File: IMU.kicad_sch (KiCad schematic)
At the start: 0 parts

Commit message: new update
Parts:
- added C29, C30: 100nF, C0402C104K4RAC:CAPC1005X55N, symbol C0402C104K4RAC:C0402C104K4RAC
- added U1: BMI088, Module:PQFN50P450X300X100-16N, symbol BMI088:BMI088
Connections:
- new net +3V3_BMI: C29.2, C30.2, U1.11 (VDDIO), U1.3 (VDD)
- new net CSB_ACCEL: U1.14 (CSB1)
- new net CSB_GYRO: U1.5 (CSB2)
- new net GND: C29.1, C30.1, U1.2 (NC), U1.4 (GNDA), U1.6 (GNDIO), U1.7 (PS)
- new net INT1_ACCEL: U1.16 (INT1)
- new net INT1_GYRO: U1.12 (INT3)
- new net INT2_ACCEL: U1.1 (INT2)
- new net INT2_GYRO: U1.13 (INT4)
- new net MISO: U1.10 (SDO2), U1.15 (SDO1)
- new net MOSI: U1.9 (SDA/SDI)
- new net SCK: U1.8 (SCL/SCK)

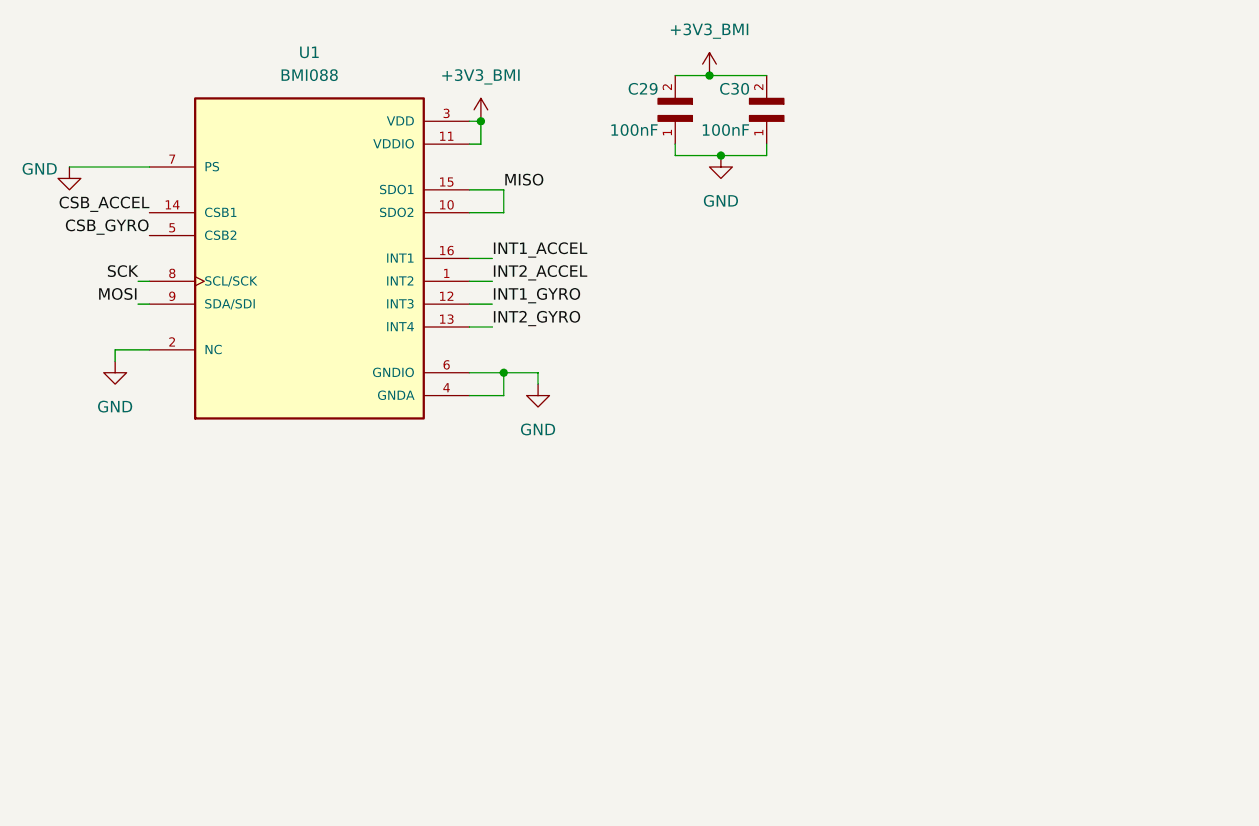
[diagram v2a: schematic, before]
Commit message: new
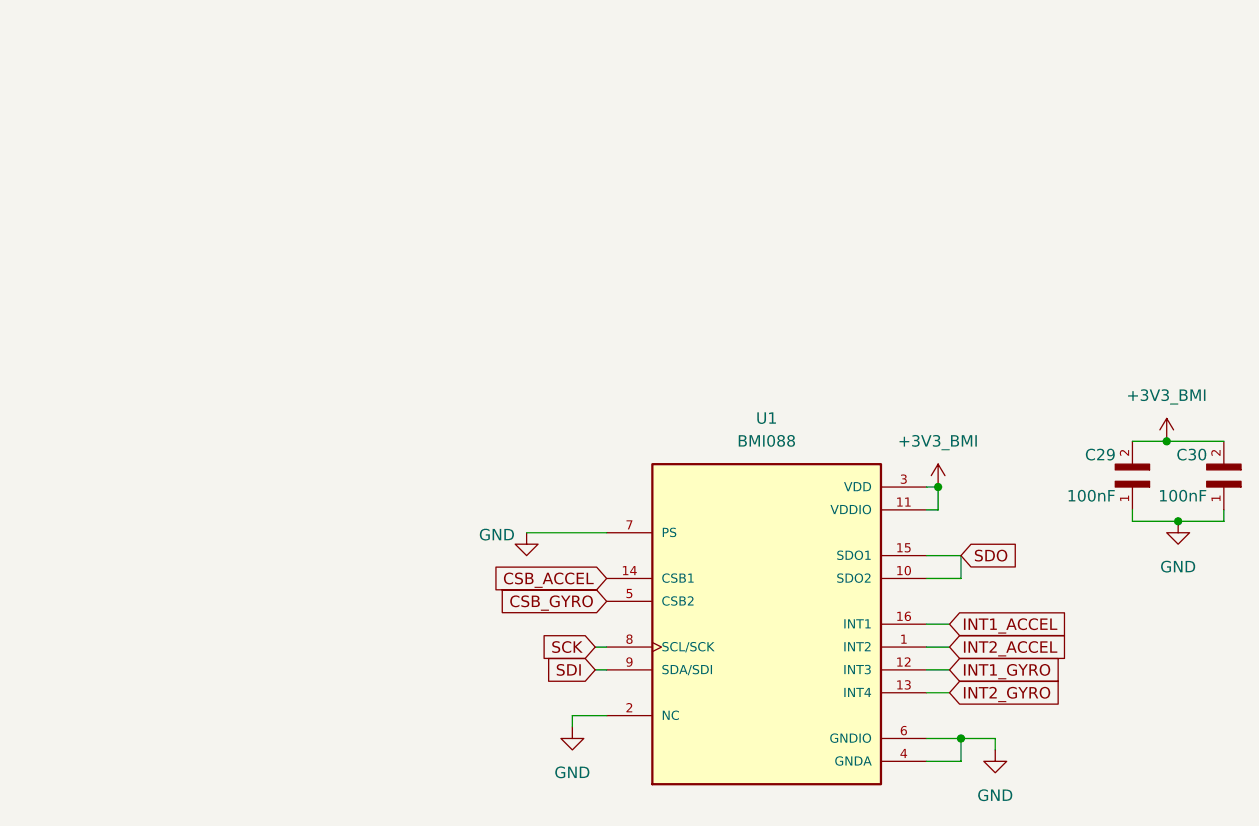
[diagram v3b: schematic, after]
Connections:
- net MISO renamed SDO
- net MOSI renamed SDI
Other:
- moved on the sheet: C29, C30, U1
